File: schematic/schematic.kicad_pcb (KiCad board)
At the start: 2 copper layers, 40.6 x 70.5 mm, 59 parts, among them J2 USB_C_Receptacle_USB2.0, J3 Pelt, J4 Serial, SW1 PS, U1 ESP32-D-WD-V3, U2 IRS2103, U3 BUK9K52-60E, U4 BUK9K52-60E, U5 IRS2103, U6 MC34063AD, U7 TP4054, Y1 Crystal_GND24

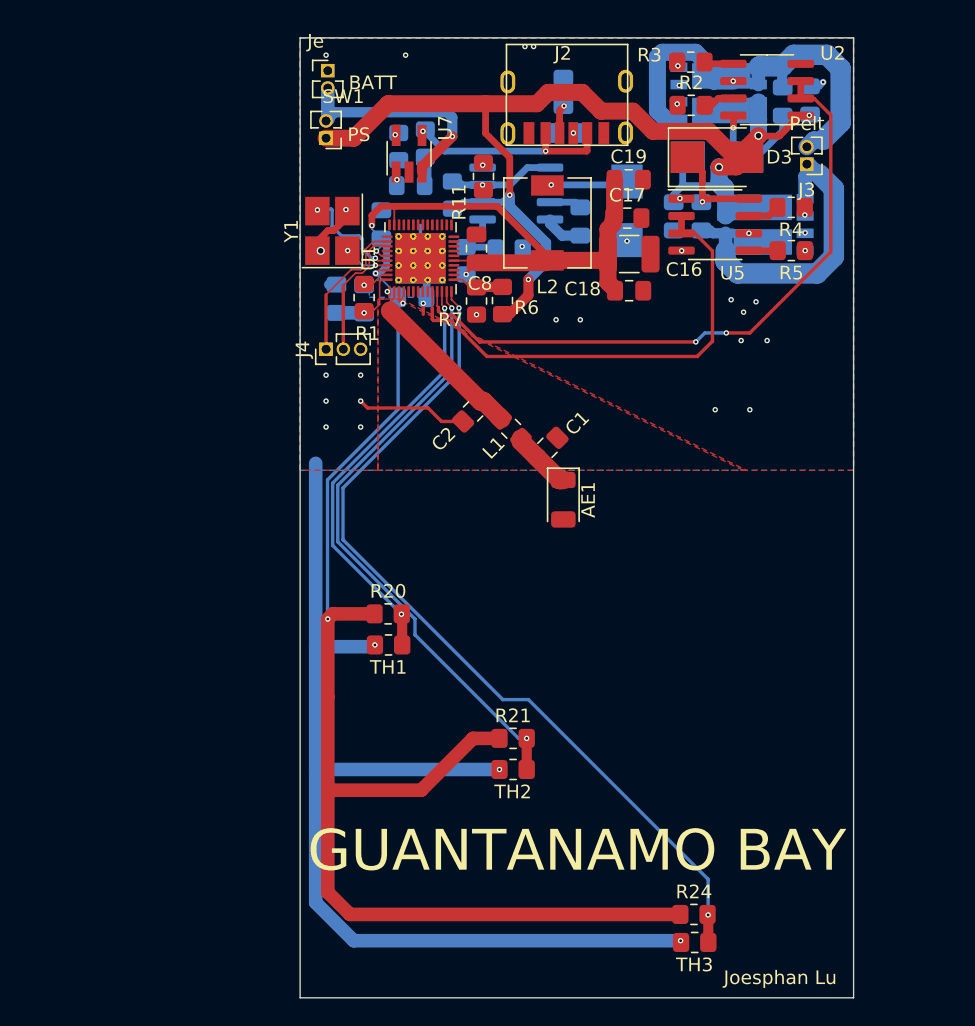
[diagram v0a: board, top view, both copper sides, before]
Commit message: final winter qtr push
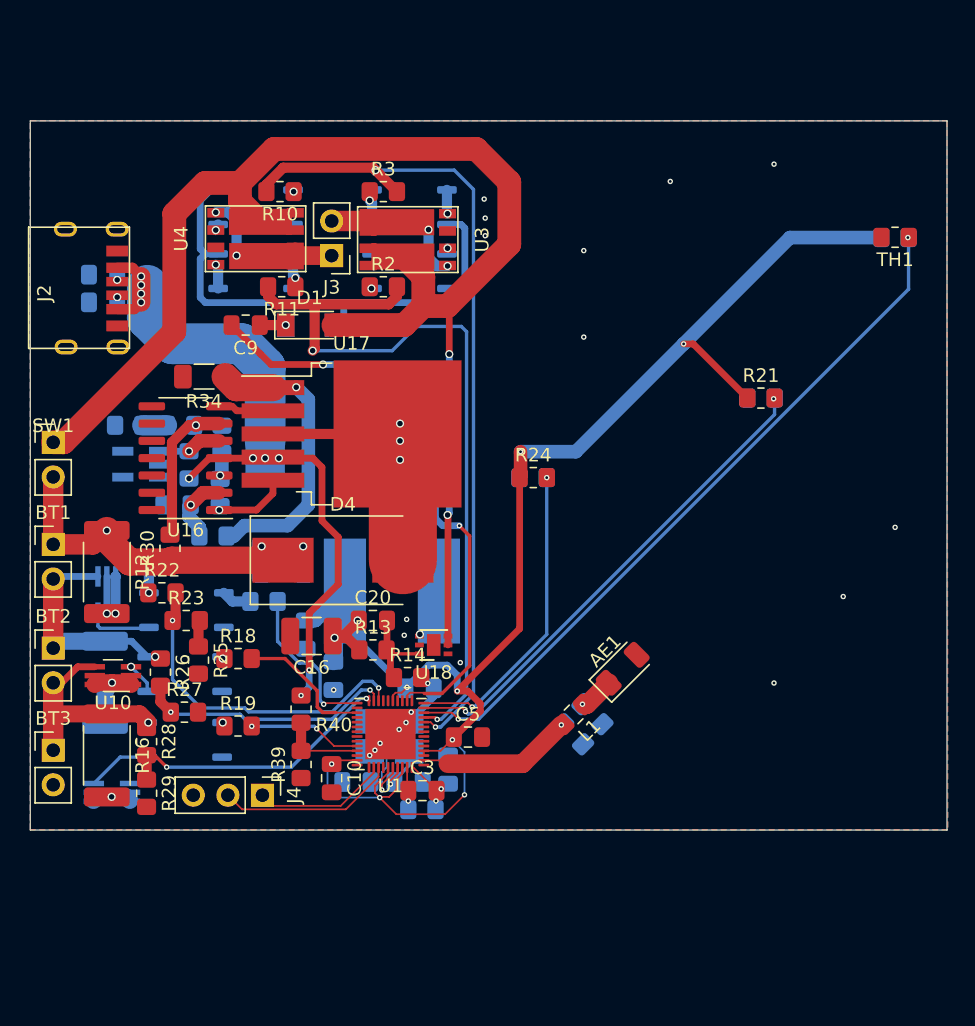
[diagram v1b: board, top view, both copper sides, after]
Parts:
- removed C12, C13, C14: 10uF, Capacitor_SMD:C_0805_2012Metric_Pad1.18x1.45mm_HandSolder
- removed C19: 100nF, Capacitor_SMD:C_0805_2012Metric_Pad1.18x1.45mm_HandSolder
- removed D3: STPS130U, Diode_SMD:D_SMB
- removed Je: BATT, Connector_PinHeader_1.27mm:PinHeader_1x02_P1.27mm_Vertical
- removed R4, R5: 10k, Resistor_SMD:R_0805_2012Metric_Pad1.20x1.40mm_HandSolder
- removed R6: 76k, Resistor_SMD:R_0805_2012Metric_Pad1.20x1.40mm_HandSolder
- removed R7: 24k, Resistor_SMD:R_0805_2012Metric_Pad1.20x1.40mm_HandSolder
- removed U5: IRS2103, Package_SO:SOIC-8_3.9x4.9mm_P1.27mm
- added BT1: Battery_Cell, Connector_PinHeader_2.54mm:PinHeader_1x02_P2.54mm_Vertical, F.Cu at (117.3, 99.0)
- added BT2: Battery_Cell, Connector_PinHeader_2.54mm:PinHeader_1x02_P2.54mm_Vertical, F.Cu at (117.3, 106.7)
- added BT3: Battery_Cell, Connector_PinHeader_2.54mm:PinHeader_1x02_P2.54mm_Vertical, F.Cu at (117.3, 114.2)
- added C20: Cfw (DNP), Capacitor_SMD:C_0805_2012Metric_Pad1.18x1.45mm_HandSolder, F.Cu at (140.7, 104.6)
- added C21: 100nF, Capacitor_SMD:C_0805_2012Metric_Pad1.18x1.45mm_HandSolder, B.Cu at (132.6, 100.2)
- added C9: 10uF, Capacitor_SMD:C_0805_2012Metric_Pad1.18x1.45mm_HandSolder, F.Cu at (131.4, 82.9)
- added L3: 33uH, Inductor_SMD:L_12x12mm_H4.5mm, B.Cu at (137.8, 91.4)
- added R16: 28.7, Resistor_SMD:R_2512_6332Metric_Pad1.40x3.35mm_HandSolder, F.Cu at (121.2, 114.5)
- added R17: 200, Resistor_SMD:R_0805_2012Metric_Pad1.20x1.40mm_HandSolder, B.Cu at (132.7, 103.2)
- added R18: 200, Resistor_SMD:R_0805_2012Metric_Pad1.20x1.40mm_HandSolder, F.Cu at (130.8, 107.4)
- added R19: 200, Resistor_SMD:R_0805_2012Metric_Pad1.20x1.40mm_HandSolder, F.Cu at (130.8, 112.4)
- added R22: 100k, Resistor_SMD:R_0805_2012Metric_Pad1.20x1.40mm_HandSolder, F.Cu at (125.2, 102.6)
- added R23: 22k, Resistor_SMD:R_0805_2012Metric_Pad1.20x1.40mm_HandSolder, F.Cu at (127.0, 104.6)
- added R25: 390, Resistor_SMD:R_0805_2012Metric_Pad1.20x1.40mm_HandSolder, F.Cu at (127.9, 107.5)
- added R26: 180k, Resistor_SMD:R_0805_2012Metric_Pad1.20x1.40mm_HandSolder, F.Cu at (125.1, 108.4)
- added R27: 68k, Resistor_SMD:R_0805_2012Metric_Pad1.20x1.40mm_HandSolder, F.Cu at (126.9, 111.4)
- added R28: 56k, Resistor_SMD:R_0805_2012Metric_Pad1.20x1.40mm_HandSolder, F.Cu at (124.1, 113.5)
- added R29: 68k, Resistor_SMD:R_0805_2012Metric_Pad1.20x1.40mm_HandSolder, F.Cu at (124.1, 117.3)
- added R30: 220k, Resistor_SMD:R_0805_2012Metric_Pad1.20x1.40mm_HandSolder, F.Cu at (125.8, 99.3)
- added R31: 56k, Resistor_SMD:R_0805_2012Metric_Pad1.20x1.40mm_HandSolder, B.Cu at (126.6, 90.3)
- added R32: 120, Resistor_SMD:R_0805_2012Metric_Pad1.20x1.40mm_HandSolder, B.Cu at (122.8, 90.3)
- added R33: 500, Resistor_SMD:R_0805_2012Metric_Pad1.20x1.40mm_HandSolder, B.Cu at (127.2, 93.2)
- added R34: .1, Resistor_SMD:R_1206_3216Metric_Pad1.30x1.75mm_HandSolder, F.Cu at (128.3, 86.7)
- added R35: 1k, Resistor_SMD:R_0805_2012Metric_Pad1.20x1.40mm_HandSolder, B.Cu at (129.0, 98.4)
- added R36: 1k, Resistor_SMD:R_0805_2012Metric_Pad1.20x1.40mm_HandSolder, B.Cu at (129.6, 91.3)
- added R37: 12.5k, Resistor_SMD:R_0805_2012Metric_Pad1.20x1.40mm_HandSolder, B.Cu at (126.3, 96.1)
- added R38: 12.5k, Resistor_SMD:R_0805_2012Metric_Pad1.20x1.40mm_HandSolder, B.Cu at (129.5, 95.2)
- added R39: 150k, Resistor_SMD:R_0805_2012Metric_Pad1.20x1.40mm_HandSolder, F.Cu at (135.5, 115.2)
- added R40: 100k, Resistor_SMD:R_0805_2012Metric_Pad1.20x1.40mm_HandSolder, F.Cu at (135.5, 111.1)
- added U10: BSD316, Package_TO_SOT_SMD:SOT-363_SC-70-6_Handsoldering, F.Cu at (121.6, 108.7)
- added U11: BSD316, Package_TO_SOT_SMD:SOT-363_SC-70-6_Handsoldering, B.Cu at (121.6, 117.2)
- added U12: PC817, Package_SO:SOP-4_3.8x4.1mm_P2.54mm, B.Cu at (127.0, 103.9)
- added U13: PC817, Package_SO:SOP-4_3.8x4.1mm_P2.54mm, B.Cu at (126.9, 108.6)
- added U14: PC817, Package_SO:SOP-4_3.8x4.1mm_P2.54mm, B.Cu at (126.9, 113.4)
- added U15: AS431, Package_TO_SOT_SMD:SOT-23-5_HandSoldering, B.Cu at (123.7, 93.2)
- added U16: LM324, Package_SO:SOIC-14_3.9x8.7mm_P1.27mm, F.Cu at (127.0, 92.7)
- added U17: XL6009, Package_TO_SOT_SMD:TO-263-5_TabPin3, F.Cu at (139.2, 90.9)
- added U18: PAM2305CGFADJ, Package_DFN_QFN:DFN-6-1EP_2x2mm_P0.65mm_EP1x1.6mm, F.Cu at (145.2, 106.4)
- added U8: PC817, Package_SO:SOP-4_3.8x4.1mm_P2.54mm, B.Cu at (132.1, 79.0)
- added U9: BSD316, Package_TO_SOT_SMD:SOT-363_SC-70-6_Handsoldering, B.Cu at (121.2, 102.7)
- C1, C17, C18, C2, C8, R1, R20, TH2, TH3, Y1: moved to B.Cu
- C10, C3, C5, U3, U4: moved to F.Cu
- C15: value 100pF -> 10uF
- D1: value STPS130U -> LL4148; footprint Diode_SMD:D_SMB -> Diode_SMD:D_MiniMELF; moved to F.Cu
- D2: value STPS130U -> LL4148; footprint Diode_SMD:D_SMB -> Diode_SMD:D_MiniMELF
- D4: value LED -> SS34; footprint LED_SMD:LED_0805_2012Metric_Pad1.15x1.40mm_HandSolder -> Diode_SMD:D_SMC_Handsoldering; moved to F.Cu
- J3: value Pelt -> Peltier Connection; footprint Connector_PinHeader_1.27mm:PinHeader_1x02_P1.27mm_Vertical -> Connector_PinHeader_2.54mm:PinHeader_1x02_P2.54mm_Vertical
- J4: footprint Connector_PinHeader_1.27mm:PinHeader_1x03_P1.27mm_Vertical -> Connector_PinHeader_2.54mm:PinHeader_1x03_P2.54mm_Vertical
- L2: value 150uH -> 10uH NR8040T100M; footprint Inductor_SMD:L_6.3x6.3_H3 -> Inductor_SMD:L_Taiyo-Yuden_NR-80xx_HandSoldering; moved to B.Cu
- R10: value .22 -> 300; moved to F.Cu
- R11: value 180 -> 300
- R12: value 500 -> 28.7; footprint Resistor_SMD:R_0805_2012Metric_Pad1.20x1.40mm_HandSolder -> Resistor_SMD:R_2512_6332Metric_Pad1.40x3.35mm_HandSolder; moved to F.Cu
- R13: value 3.6k -> 33k; moved to F.Cu
- R14: value 2.2k -> 7.5k; moved to F.Cu
- R15: value 470 -> 28.7; footprint Resistor_SMD:R_0805_2012Metric_Pad1.20x1.40mm_HandSolder -> Resistor_SMD:R_2512_6332Metric_Pad1.40x3.35mm_HandSolder
- R2, R3: value 10k -> 300
- SW1: value PS -> Power Switch; footprint Connector_PinHeader_1.27mm:PinHeader_1x02_P1.27mm_Vertical -> Connector_PinHeader_2.54mm:PinHeader_1x02_P2.54mm_Vertical
- U1: footprint Package_DFN_QFN:QFN-48-1EP_5x5mm_P0.35mm_EP3.7x3.7mm_ThermalVias -> Package_DFN_QFN:QFN-48-1EP_5x5mm_P0.35mm_EP3.7x3.7mm
- U2: value IRS2103 -> PC817; footprint Package_SO:SOIC-8_3.9x4.9mm_P1.27mm -> Package_SO:SOP-4_3.8x4.1mm_P2.54mm; moved to B.Cu
- U6: value MC34063AD -> PC817; footprint Package_SO:SOIC-8_3.9x4.9mm_P1.27mm -> Package_SO:SOP-4_3.8x4.1mm_P2.54mm
- U7: value TP4054 -> PC817; footprint Package_TO_SOT_SMD:SOT-23-5_HandSoldering -> Package_SO:SOP-4_3.8x4.1mm_P2.54mm; moved to B.Cu
- moved TH1 47.7 mm to (179.1, 76.5)
- moved R20 46.3 mm to (179.1, 76.5)
- moved R15 46.1 mm to (121.1, 109.2)
- moved C7 42.1 mm to (139.5, 116.5), turned to 180 degrees
- moved C10 40.8 mm to (137.7, 116.2), turned to -90 degrees
- moved U4 40.5 mm to (130.6, 79.8)
- moved C6 39.4 mm to (143.3, 116.5), turned to 0 degrees
- moved C17 38.6 mm to (135.8, 105.7), turned to -90 degrees
- moved R12 37.9 mm to (121.2, 101.1), turned to -90 degrees
- moved R1 37.8 mm to (144.3, 118.5), turned to 0 degrees
- moved Y1 37.4 mm to (141.9, 113.1), turned to 180 degrees
- moved R8 37.2 mm to (120.9, 81.3), turned to 180 degrees
- moved C16 36.5 mm to (136.2, 105.8), turned to 180 degrees
- moved C3 36.3 mm to (144.4, 117.1), turned to 0 degrees
- moved TH3 36.1 mm to (152.5, 94.1)
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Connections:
- AE1 pad 2: Net-(AE1-Pad2) -> unconnected-(AE1-Pad2)
- C11 pad 1: VCC_UNREGULATED -> Vdrive
- C15 pad 1: Net-(C15-Pad1) -> +BATT
- D1 pad 1: Net-(C12-Pad1) -> Net-(C9-Pad1)
- D2 pad 1: Net-(D2-Pad1) -> Vdrive
- D2 pad 2: GND -> Net-(C9-Pad1)
- D4 pad 1: Net-(D4-Pad1) -> +BATT
- J2 pad A9: VBUS -> USB_PWR
- J2 pad B9: VBUS -> USB_PWR
- L2 pad 2: Net-(D2-Pad1) -> Net-(L2-Pad2)
- R10 pad 2: VCC_UNREGULATED -> DRIVER_N
- R11 pad 1: Net-(R10-Pad1) -> Net-(R11-Pad1)
- R11 pad 2: Net-(R11-Pad2) -> DRIVER_P
- R12 pad 1: GND -> +BATT
- R15 pad 1: VBUS -> Net-(BT1-Pad2)
- R15 pad 2: Net-(D4-Pad2) -> Net-(R15-Pad2)
- R2 pad 2: Net-(R2-Pad2) -> DRIVER_P
- R3 pad 2: Net-(R3-Pad2) -> DRIVER_N
- SW1 pad 2: /Power Management/BATT_IN -> +BATT
- U1 pad 15: Net-(R6-Pad2) -> unconnected-(U1-Pad15)
- U1 pad 16: Net-(U1-Pad16) -> PWM
- U1 pad 17: Net-(U1-Pad17) -> unconnected-(U1-Pad17)
- U1 pad 18: Net-(U1-Pad18) -> unconnected-(U1-Pad18)
- U1 pad 20: Net-(U1-Pad20) -> unconnected-(U1-Pad20)
- U1 pad 21: Net-(U1-Pad21) -> unconnected-(U1-Pad21)
- U1 pad 22: Net-(U1-Pad22) -> CELL_MEAS_3
- U1 pad 23: Net-(U1-Pad23) -> CELL_MEAS_2
- U1 pad 24: Net-(U1-Pad24) -> CELL_MEAS_1
- U1 pad 25: Net-(U1-Pad25) -> CELL_DSCHG_3
- U1 pad 26: Net-(U1-Pad26) -> unconnected-(U1-Pad26)
- U1 pad 27: Net-(U1-Pad27) -> CELL_DSCHG_2
- U1 pad 28: Net-(U1-Pad28) -> unconnected-(U1-Pad28)
- U1 pad 29: Net-(U1-Pad29) -> unconnected-(U1-Pad29)
- U1 pad 30: Net-(U1-Pad30) -> unconnected-(U1-Pad30)
- U1 pad 31: Net-(U1-Pad31) -> unconnected-(U1-Pad31)
- U1 pad 32: Net-(U1-Pad32) -> unconnected-(U1-Pad32)
- U1 pad 33: Net-(U1-Pad33) -> unconnected-(U1-Pad33)
- U1 pad 34: Net-(U1-Pad34) -> CELL_DSCHG_1
- U1 pad 36: Net-(U1-Pad36) -> unconnected-(U1-Pad36)
- U1 pad 38: Net-(U1-Pad38) -> unconnected-(U1-Pad38)
- U1 pad 39: Net-(U1-Pad39) -> unconnected-(U1-Pad39)
- U1 pad 42: Net-(U1-Pad42) -> unconnected-(U1-Pad42)
- U1 pad 5: Net-(U1-Pad5) -> unconnected-(U1-Pad5)
- U1 pad 6: Net-(U1-Pad6) -> unconnected-(U1-Pad6)
- U1 pad 7: Net-(U1-Pad7) -> unconnected-(U1-Pad7)
- U1 pad 8: Net-(U1-Pad8) -> unconnected-(U1-Pad8)
- U1 pad 9: Net-(U1-Pad9) -> unconnected-(U1-Pad9)
- U2 pad 1: VCC_UNREGULATED -> Net-(R2-Pad1)
- U2 pad 2: DRIVER_P -> GND
- U2 pad 3: DRIVER_P -> Net-(U3-Pad2)
- U2 pad 4: GND -> unconnected-(U2-Pad4)
- U3 pad 2: Net-(R2-Pad1) -> Net-(U3-Pad2)
- U3 pad 4: Net-(R3-Pad1) -> Net-(U3-Pad4)
- U4 pad 2: Net-(R4-Pad1) -> Net-(U4-Pad2)
- U6 pad 1: Net-(R10-Pad1) -> Net-(R3-Pad1)
- U6 pad 2: Net-(D2-Pad1) -> GND
- U6 pad 3: Net-(C15-Pad1) -> Net-(U3-Pad4)
- U6 pad 4: GND -> Vdrive
- U7 pad 1: Net-(D4-Pad1) -> Net-(R10-Pad1)
- U7 pad 3: /Power Management/BATT_IN -> Net-(U4-Pad2)
- U7 pad 4: VBUS -> Vdrive
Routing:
- net GND: track 102.3 -> 3.18 mm, vias 32 -> 21
- net USB_PWR: track 0.00 -> 54.7 mm, vias 0 -> 10
- net PWM: track 0.00 -> 44.9 mm, vias 0 -> 2
- net TEMP_SENSE_3: track 63.8 -> 22.9 mm
- net Vdrive: track 0.00 -> 39.5 mm
- net +BATT: track 0.00 -> 29.5 mm, vias 0 -> 4
- net DRIVER_N: track 34.9 -> 61.0 mm, vias 0 -> 2
- net /Peltier Driver/PELTIER_P: track 31.6 -> 6.37 mm, vias 1 -> 2
- net CELL_MEAS_3: track 0.00 -> 24.7 mm, vias 0 -> 2
- net +3V3: track 141.9 -> 117.4 mm, vias 7 -> 10
- net Net-(R34-Pad1): track 0.00 -> 21.5 mm, vias 0 -> 1
- net TEMP_SENSE_1: track 31.6 -> 52.7 mm
- net CELL_MEAS_1: track 0.00 -> 20.6 mm, vias 0 -> 2
- net VCC_UNREGULATED: track 80.6 -> 101.2 mm, vias 6 -> 2
- net CELL_MEAS_2: track 0.00 -> 19.0 mm, vias 0 -> 2
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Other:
- board size 40.6 x 70.5 mm -> 67.3 x 52.1 mm
- net class Default removed
